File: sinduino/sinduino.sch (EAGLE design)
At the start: 22 parts, among them IC1 IC_UC_ATMEGA32U4-TQFP44, Q1 16000, X1 MINI-USB-32005-301

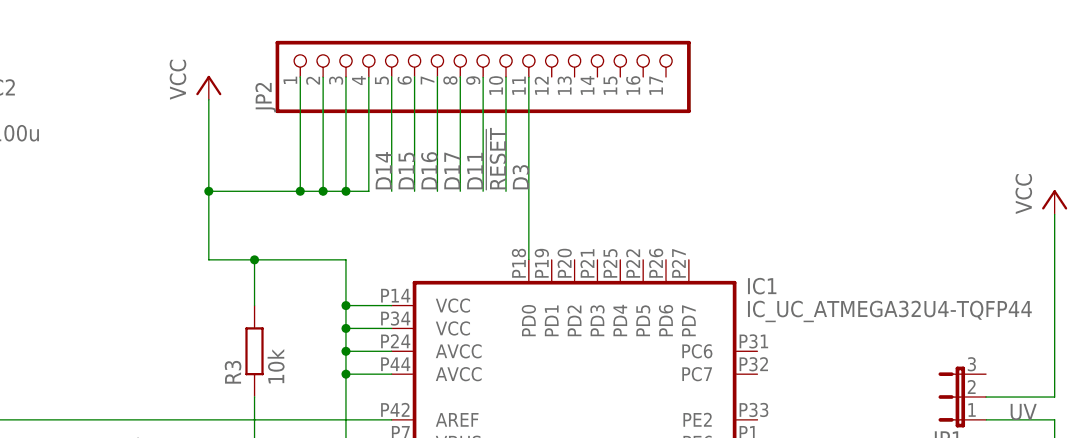
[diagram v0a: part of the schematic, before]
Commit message: proceed connecting
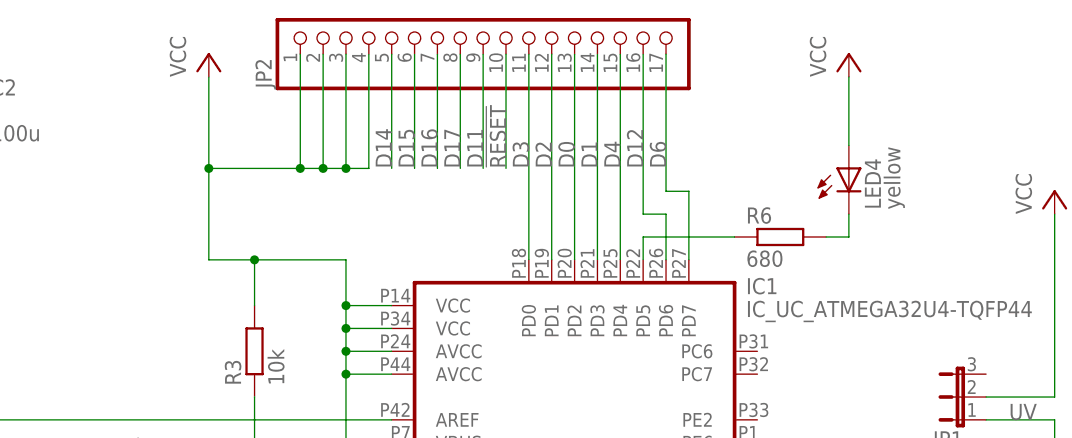
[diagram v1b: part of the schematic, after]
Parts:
- added LED4: yellow, led:LED3MM
- added R6: 680, rcl:R-EU_R1206
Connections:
- new net D0: IC1.PD2, JP2.13
- new net D1: IC1.PD3, JP2.14
- new net D12: IC1.PD6, JP2.16
- new net D2: IC1.PD1, JP2.12
- new net D4: IC1.PD4, JP2.15
- new net D6: IC1.PD7, JP2.17
- new net N$11: LED4.C, R6.2
- new net N$2: IC1.PD5, R6.1
- net VCC: now also LED4.A
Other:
- moved on the sheet: JP2
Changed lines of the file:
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@@
 <part name="P+5" library="supply1" deviceset="VCC" device=""/>
 <part name="GND10" library="supply1" deviceset="GND" device=""/>
+<part name="R6" library="rcl" deviceset="R-EU_" device="R1206" value="680"/>
+<part name="LED4" library="led" deviceset="LED" device="3MM" value="yellow"/>
+<part name="P+1" library="supply1" deviceset="VCC" device=""/>
 </parts>
 <sheets>
@@
 <instance part="JP1" gate="1" x="109.22" y="73.66" rot="R90"/>
 <instance part="P+4" gate="VCC" x="119.38" y="96.52"/>
-<instance part="JP2" gate="G$1" x="53.34" y="111.76" rot="R90"/>
+<instance part="JP2" gate="G$1" x="53.34" y="114.3" rot="R90"/>
 <instance part="JP3" gate="G$1" x="83.82" y="7.62" rot="R270"/>
-<instance part="P+5" gate="VCC" x="25.4" y="109.22"/>
+<instance part="P+5" gate="VCC" x="25.4" y="111.76"/>
 <instance part="GND10" gate="1" x="55.88" y="-5.08"/>
+<instance part="R6" gate="G$1" x="88.9" y="91.44"/>
+<instance part="LED4" gate="G$1" x="96.52" y="99.06"/>
+<instance part="P+1" gate="VCC" x="96.52" y="111.76"/>
 </instances>
 <busses>
@@
 <segment>
 <pinref part="JP2" gate="G$1" pin="1"/>
-<wire x1="35.56" y1="109.22" x2="35.56" y2="96.52" width="0.1524" layer="91"/>
+<wire x1="35.56" y1="111.76" x2="35.56" y2="99.06" width="0.1524" layer="91"/>
 <pinref part="JP2" gate="G$1" pin="4"/>
-<wire x1="43.18" y1="109.22" x2="43.18" y2="96.52" width="0.1524" layer="91"/>
-<wire x1="43.18" y1="96.52" x2="40.64" y2="96.52" width="0.1524" layer="91"/>
-<wire x1="40.64" y1="96.52" x2="38.1" y2="96.52" width="0.1524" layer="91"/>
-<wire x1="38.1" y1="96.52" x2="35.56" y2="96.52" width="0.1524" layer="91"/>
-<wire x1="35.56" y1="96.52" x2="25.4" y2="96.52" width="0.1524" layer="91"/>
-<wire x1="25.4" y1="96.52" x2="25.4" y2="106.68" width="0.1524" layer="91"/>
-<junction x="35.56" y="96.52"/>
+<wire x1="43.18" y1="111.76" x2="43.18" y2="99.06" width="0.1524" layer="91"/>
+<wire x1="43.18" y1="99.06" x2="40.64" y2="99.06" width="0.1524" layer="91"/>
+<wire x1="40.64" y1="99.06" x2="38.1" y2="99.06" width="0.1524" layer="91"/>
+<wire x1="38.1" y1="99.06" x2="35.56" y2="99.06" width="0.1524" layer="91"/>
+<wire x1="35.56" y1="99.06" x2="25.4" y2="99.06" width="0.1524" layer="91"/>
+<wire x1="25.4" y1="99.06" x2="25.4" y2="109.22" width="0.1524" layer="91"/>
+<junction x="35.56" y="99.06"/>
 <pinref part="JP2" gate="G$1" pin="2"/>
-<wire x1="38.1" y1="109.22" x2="38.1" y2="96.52" width="0.1524" layer="91"/>
-<junction x="38.1" y="96.52"/>
+<wire x1="38.1" y1="111.76" x2="38.1" y2="99.06" width="0.1524" layer="91"/>
+<junction x="38.1" y="99.06"/>
 <pinref part="JP2" gate="G$1" pin="3"/>
-<wire x1="40.64" y1="109.22" x2="40.64" y2="96.52" width="0.1524" layer="91"/>
-<junction x="40.64" y="96.52"/>
+<wire x1="40.64" y1="111.76" x2="40.64" y2="99.06" width="0.1524" layer="91"/>
+<junction x="40.64" y="99.06"/>
 <pinref part="P+5" gate="VCC" pin="VCC"/>
-<wire x1="25.4" y1="96.52" x2="25.4" y2="88.9" width="0.1524" layer="91"/>
+<wire x1="25.4" y1="99.06" x2="25.4" y2="88.9" width="0.1524" layer="91"/>
 <pinref part="R3" gate="G$1" pin="2"/>
 <wire x1="30.48" y1="83.82" x2="30.48" y2="88.9" width="0.1524" layer="91"/>
@@
 <wire x1="30.48" y1="88.9" x2="40.64" y2="88.9" width="0.1524" layer="91"/>
 <junction x="30.48" y="88.9"/>
-<junction x="25.4" y="96.52"/>
+<junction x="25.4" y="99.06"/>
+</segment>
+<segment>
+<pinref part="LED4" gate="G$1" pin="A"/>
+<pinref part="P+1" gate="VCC" pin="VCC"/>
+<wire x1="96.52" y1="101.6" x2="96.52" y2="109.22" width="0.1524" layer="91"/>
 </segment>
 </net>
@@
 <segment>
 <pinref part="JP2" gate="G$1" pin="10"/>
-<wire x1="58.42" y1="109.22" x2="58.42" y2="96.52" width="0.1524" layer="91"/>
-<label x="58.42" y="96.52" size="1.778" layer="95" rot="R90"/>
+<wire x1="58.42" y1="111.76" x2="58.42" y2="99.06" width="0.1524" layer="91"/>
+<label x="58.42" y="99.06" size="1.778" layer="95" rot="R90"/>
 </segment>
 </net>
@@
 <segment>
 <pinref part="JP2" gate="G$1" pin="5"/>
-<wire x1="45.72" y1="109.22" x2="45.72" y2="96.52" width="0.1524" layer="91"/>
-<label x="45.72" y="96.52" size="1.778" layer="95" rot="R90"/>
+<wire x1="45.72" y1="111.76" x2="45.72" y2="99.06" width="0.1524" layer="91"/>
+<label x="45.72" y="99.06" size="1.778" layer="95" rot="R90"/>
 </segment>
 </net>
@@
 <segment>
 <pinref part="JP2" gate="G$1" pin="6"/>
-<wire x1="48.26" y1="109.22" x2="48.26" y2="96.52" width="0.1524" layer="91"/>
-<label x="48.26" y="96.52" size="1.778" layer="95" rot="R90"/>
+<wire x1="48.26" y1="111.76" x2="48.26" y2="99.06" width="0.1524" layer="91"/>
+<label x="48.26" y="99.06" size="1.778" layer="95" rot="R90"/>
 </segment>
 <segment>
@@
 <segment>
 <pinref part="JP2" gate="G$1" pin="7"/>
-<wire x1="50.8" y1="109.22" x2="50.8" y2="96.52" width="0.1524" layer="91"/>
-<label x="50.8" y="96.52" size="1.778" layer="95" rot="R90"/>
+<wire x1="50.8" y1="111.76" x2="50.8" y2="99.06" width="0.1524" layer="91"/>
+<label x="50.8" y="99.06" size="1.778" layer="95" rot="R90"/>
 </segment>
 <segment>
@@
 <segment>
 <pinref part="JP2" gate="G$1" pin="8"/>
-<wire x1="53.34" y1="109.22" x2="53.34" y2="96.52" width="0.1524" layer="91"/>
-<label x="53.34" y="96.52" size="1.778" layer="95" rot="R90"/>
+<wire x1="53.34" y1="111.76" x2="53.34" y2="99.06" width="0.1524" layer="91"/>
+<label x="53.34" y="99.06" size="1.778" layer="95" rot="R90"/>
 </segment>
 <segment>
@@
 <segment>
 <pinref part="JP2" gate="G$1" pin="9"/>
-<wire x1="55.88" y1="109.22" x2="55.88" y2="96.52" width="0.1524" layer="91"/>
-<label x="55.88" y="96.52" size="1.778" layer="95" rot="R90"/>
+<wire x1="55.88" y1="111.76" x2="55.88" y2="99.06" width="0.1524" layer="91"/>
+<label x="55.88" y="99.06" size="1.778" layer="95" rot="R90"/>
 </segment>
 </net>
@@
 <segment>
 <pinref part="JP2" gate="G$1" pin="11"/>
-<wire x1="60.96" y1="109.22" x2="60.96" y2="88.9" width="0.1524" layer="91"/>
+<wire x1="60.96" y1="111.76" x2="60.96" y2="88.9" width="0.1524" layer="91"/>
 <pinref part="IC1" gate="IC" pin="PD0"/>
-<label x="60.96" y="96.52" size="1.778" layer="95" rot="R90"/>
-</segment>
-</net>
+<label x="60.96" y="99.06" size="1.778" layer="95" rot="R90"/>
+</segment>
+</net>
+<net name="D2" class="0">
+<segment>
+<pinref part="JP2" gate="G$1" pin="12"/>
+<pinref part="IC1" gate="IC" pin="PD1"/>
+<wire x1="63.5" y1="111.76" x2="63.5" y2="88.9" width="0.1524" layer="91"/>
+<label x="63.5" y="99.06" size="1.778" layer="95" rot="R90"/>
+</segment>
+</net>
+<net name="D0" class="0">
+<segment>
+<pinref part="IC1" gate="IC" pin="PD2"/>
+<pinref part="JP2" gate="G$1" pin="13"/>
+<wire x1="66.04" y1="88.9" x2="66.04" y2="111.76" width="0.1524" layer="91"/>
+<label x="66.04" y="99.06" size="1.778" layer="95" rot="R90"/>
+</segment>
+</net>
+<net name="D1" class="0">
+<segment>
+<pinref part="IC1" gate="IC" pin="PD3"/>
+<pinref part="JP2" gate="G$1" pin="14"/>
+<wire x1="68.58" y1="88.9" x2="68.58" y2="111.76" width="0.1524" layer="91"/>
+<label x="68.58" y="99.06" size="1.778" layer="95" rot="R90"/>
+</segment>
+</net>
+<net name="D4" class="0">
+<segment>
+<pinref part="IC1" gate="IC" pin="PD4"/>
+<pinref part="JP2" gate="G$1" pin="15"/>
+<wire x1="71.12" y1="88.9" x2="71.12" y2="111.76" width="0.1524" layer="91"/>
+<label x="71.12" y="99.06" size="1.778" layer="95" rot="R90"/>
+</segment>
+</net>
+<net name="D12" class="0">
+<segment>
+<pinref part="IC1" gate="IC" pin="PD6"/>
+<wire x1="76.2" y1="88.9" x2="76.2" y2="93.98" width="0.1524" layer="91"/>
+<wire x1="76.2" y1="93.98" x2="73.66" y2="93.98" width="0.1524" layer="91"/>
+<pinref part="JP2" gate="G$1" pin="16"/>
+<wire x1="73.66" y1="93.98" x2="73.66" y2="111.76" width="0.1524" layer="91"/>
+<label x="73.66" y="99.06" size="1.778" layer="95" rot="R90"/>
+</segment>
+</net>
+<net name="D6" class="0">
+<segment>
+<pinref part="IC1" gate="IC" pin="PD7"/>
+<wire x1="78.74" y1="88.9" x2="78.74" y2="96.52" width="0.1524" layer="91"/>
+<wire x1="78.74" y1="96.52" x2="76.2" y2="96.52" width="0.1524" layer="91"/>
+<pinref part="JP2" gate="G$1" pin="17"/>
+<wire x1="76.2" y1="96.52" x2="76.2" y2="111.76" width="0.1524" layer="91"/>
+<label x="76.2" y="99.06" size="1.778" layer="95" rot="R90"/>
+</segment>
+</net>
+<net name="N$2" class="0">
+<segment>
+<pinref part="IC1" gate="IC" pin="PD5"/>
+<wire x1="73.66" y1="88.9" x2="73.66" y2="91.44" width="0.1524" layer="91"/>
+<pinref part="R6" gate="G$1" pin="1"/>
+<wire x1="73.66" y1="91.44" x2="83.82" y2="91.44" width="0.1524" layer="91"/>
+</segment>
+</net>
+<net name="N$11" class="0">
+<segment>
+<pinref part="R6" gate="G$1" pin="2"/>
+<wire x1="93.98" y1="91.44" x2="96.52" y2="91.44" width="0.1524" layer="91"/>
+<pinref part="LED4" gate="G$1" pin="C"/>
+<wire x1="96.52" y1="91.44" x2="96.52" y2="93.98" width="0.1524" layer="91"/>
+</segment>
+</net>

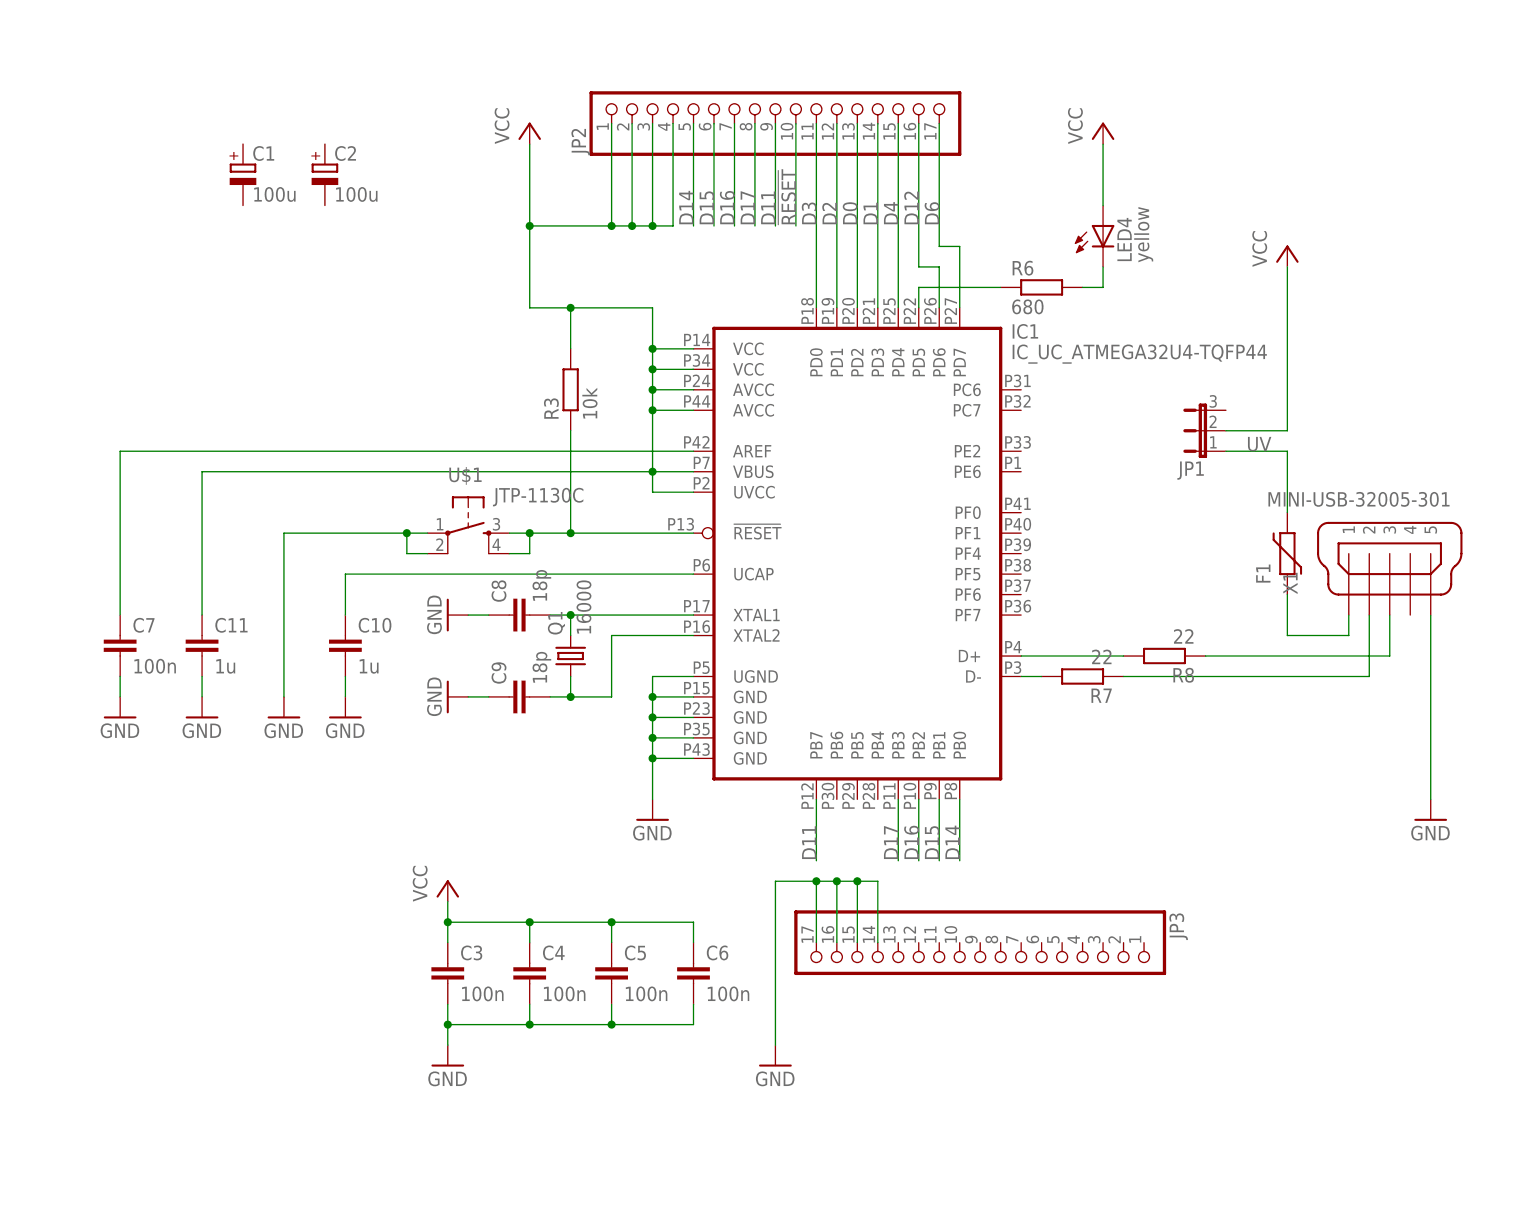
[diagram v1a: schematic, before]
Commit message: almost connected everything
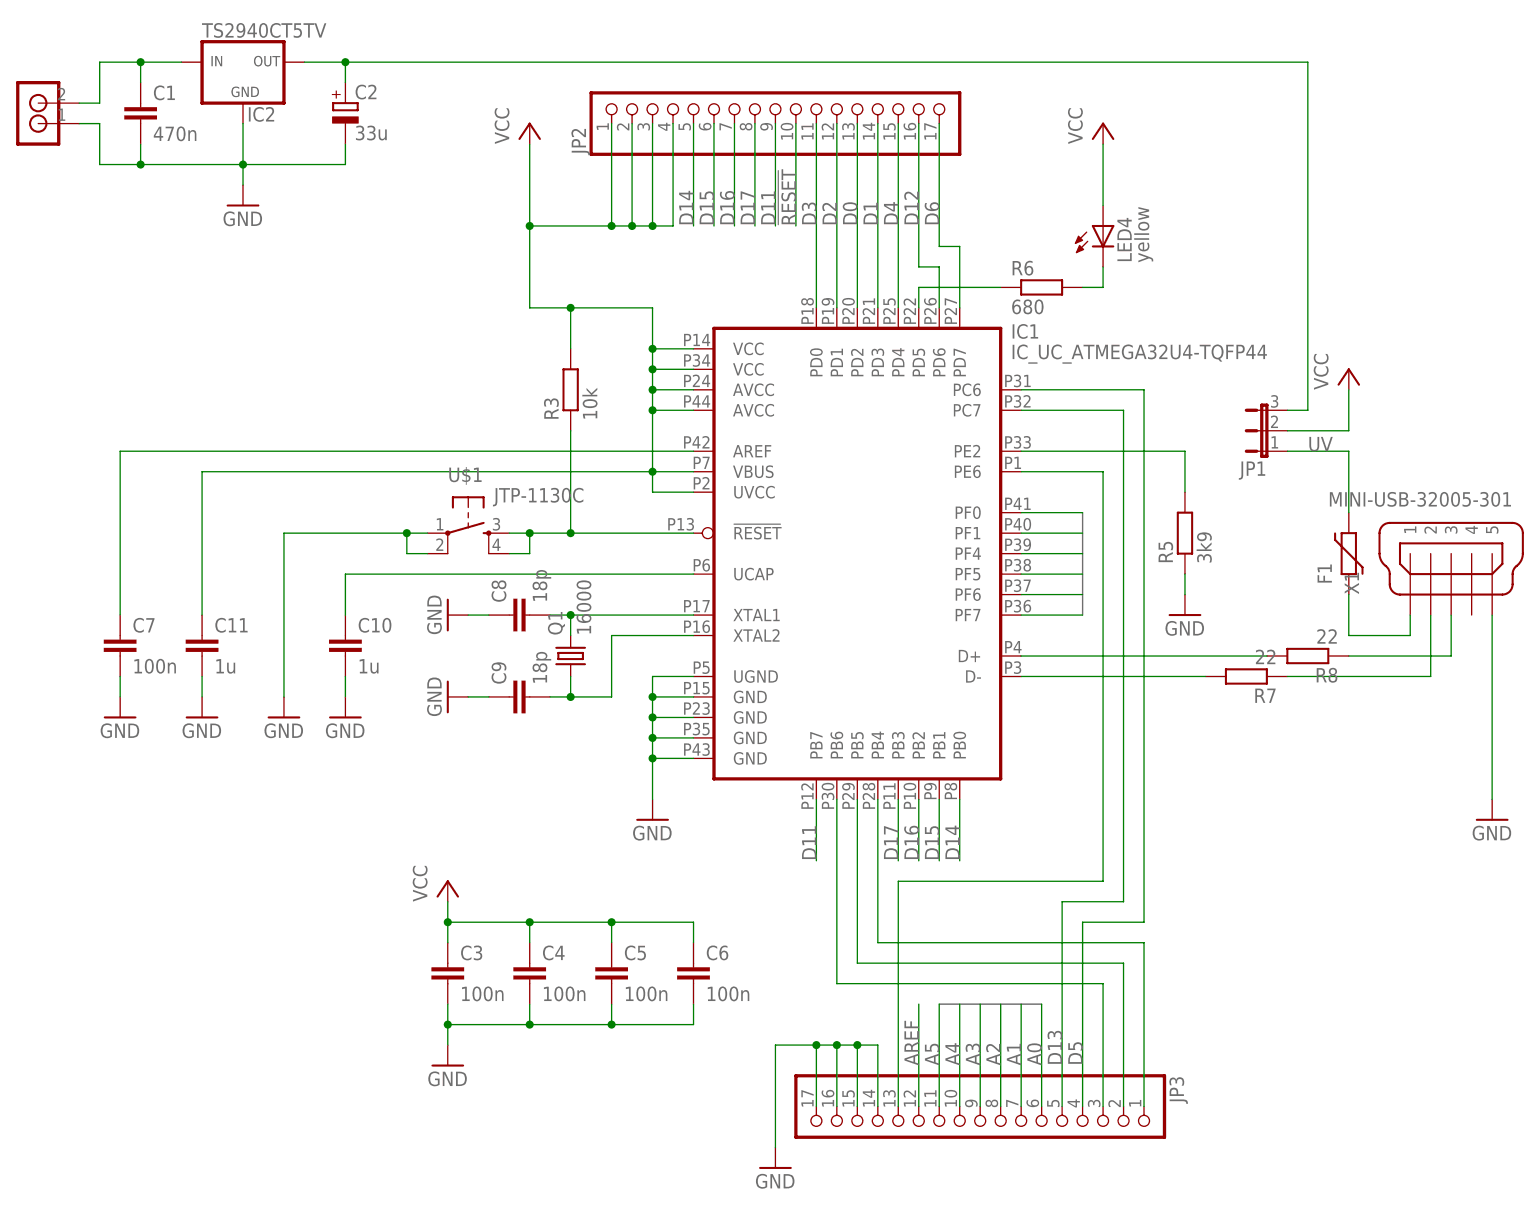
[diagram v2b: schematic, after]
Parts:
- added IC2: TS2940CT5TV, n39:TS2940CT5TV
- added R5: 3k9, rcl:R-EU_R1206
- added U$3: RIACON_101_2, n39:RIACON_101_2
- C1: value 100u -> 470n; device rcl:CPOL-EUE2.5-6 -> rcl:C-EU025-025X050
- C2: value 100u -> 33u
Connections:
- new net A0: IC1.PF7, JP3.6
- new net A1: IC1.PF6, JP3.7
- new net A2: IC1.PF5, JP3.8
- new net A3: IC1.PF4, JP3.9
- new net A4: IC1.PF1, JP3.10
- new net A5: IC1.PF0, JP3.11
- new net AREF: C7.1, IC1.AREF, JP3.12
- new net D13: IC1.PC7, JP3.5
- new net D5: IC1.PC6, JP3.4
- new net D7: IC1.PE6, JP3.13
- new net HWB: IC1.PE2, R5.2
- new net N$12: IC1.PB5, JP3.2
- new net N$13: IC1.PB4, JP3.1
- new net N$15: C1.1, IC2.IN, U$3.2
- new net N$16: C2.+, IC2.OUT, JP1.3
- net GND: now also C1.2, C2.-, IC2.GND, R5.1, U$3.1
- net N$1: now also IC1.PB6, JP3.3; no longer C7.1, IC1.AREF
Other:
- moved on the sheet: C2, F1, JP1, JP3, R7, R8, X1
